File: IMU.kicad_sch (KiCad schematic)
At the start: 5 parts, among them U12 MPU-6050

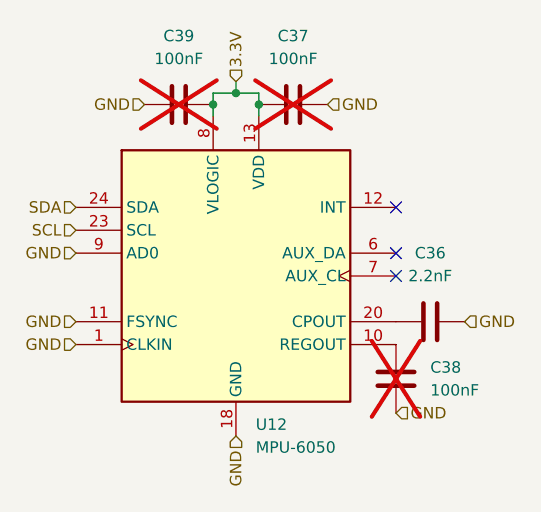
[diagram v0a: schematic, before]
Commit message: fix DNP (was just for checking what was to be bought)
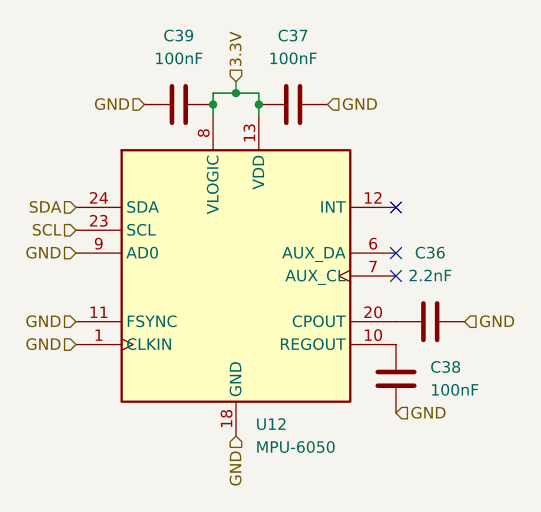
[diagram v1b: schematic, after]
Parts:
- C37, C38, C39: now fitted
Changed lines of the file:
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@@
 		(in_bom yes)
 		(on_board yes)
-		(dnp yes)
+		(dnp no)
 		(fields_autoplaced yes)
 		(property "Reference" "C39"
@@
 		(in_bom yes)
 		(on_board yes)
-		(dnp yes)
+		(dnp no)
 		(fields_autoplaced yes)
 		(property "Reference" "C37"
@@
 		(in_bom yes)
 		(on_board yes)
-		(dnp yes)
+		(dnp no)
 		(fields_autoplaced yes)
 		(property "Reference" "C38"

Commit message: update BOM + add big capas (do not take DNP into account)
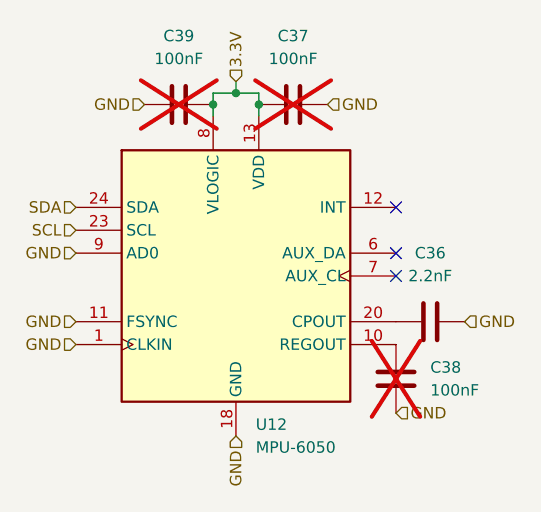
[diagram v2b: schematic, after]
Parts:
- C37, C38, C39: now not fitted
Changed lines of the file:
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@@
 		(in_bom yes)
 		(on_board yes)
-		(dnp no)
+		(dnp yes)
 		(fields_autoplaced yes)
 		(property "Reference" "C39"
@@
 		(in_bom yes)
 		(on_board yes)
-		(dnp no)
+		(dnp yes)
 		(fields_autoplaced yes)
 		(property "Reference" "C37"
@@
 		(in_bom yes)
 		(on_board yes)
-		(dnp no)
+		(dnp yes)
 		(fields_autoplaced yes)
 		(property "Reference" "C38"
